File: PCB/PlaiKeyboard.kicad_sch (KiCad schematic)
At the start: 177 parts, among them SW1 SW_Push_45deg, SW10 SW_Push_45deg, SW11 SW_Push_45deg, SW12 SW_Push_45deg, SW13 SW_Push_45deg, SW14 SW_Push_45deg, SW15 RotaryEncoder_Switch, SW16 SW_Push_45deg, SW17 SW_Push_45deg, SW18 SW_Push_45deg, SW19 SW_Push_45deg, SW2 SW_Push_45deg, SW20 SW_Push_45deg, SW21 SW_Push_45deg, SW22 SW_Push_45deg, SW23 SW_Push_45deg, SW24 SW_Push_45deg, SW25 SW_Push_45deg, SW26 SW_Push_45deg, SW27 SW_Push_45deg, SW28 SW_Push_45deg, SW29 SW_Push_45deg, SW3 SW_Push_45deg, SW30 SW_Push_45deg, SW31 SW_Push_45deg, SW32 SW_Push_45deg, SW33 SW_Push_45deg, SW34 SW_Push_45deg, SW35 SW_Push_45deg, SW36 SW_Push_45deg, SW37 SW_Push_45deg, SW38 SW_Push_45deg, SW39 SW_Push_45deg, SW4 SW_Push_45deg, SW40 SW_Push_45deg, SW41 SW_Push_45deg, SW42 SW_Push_45deg, SW43 SW_Push_45deg, SW44 SW_Push_45deg, SW45 SW_Push_45deg, SW46 SW_Push_45deg, SW47 SW_Push_45deg, SW48 SW_Push_45deg, SW49 SW_Push_45deg, SW5 SW_Push_45deg, SW50 SW_Push_45deg, SW51 SW_Push_45deg, SW52 SW_Push_45deg, SW53 SW_Push_45deg, SW54 SW_Push_45deg, SW55 SW_Push_45deg, SW56 SW_Push_45deg, SW57 SW_Push_45deg, SW58 SW_Push_45deg, SW59 SW_Push_45deg, SW6 SW_Push_45deg, SW60 SW_Push_45deg, SW61 SW_Push_45deg, SW62 SW_Push_45deg, SW63 SW_Push_45deg, SW64 SW_Push_45deg, SW65 SW_Push_45deg, SW66 SW_Push_45deg, SW67 SW_Push_45deg, SW68 SW_Push_45deg, SW69 SW_Push_45deg, SW7 SW_Push_45deg, SW70 SW_Push_45deg, SW71 SW_Push_45deg, SW72 SW_Push_45deg, SW73 SW_Push_45deg, SW74 SW_Push_45deg, SW75 SW_Push_45deg, SW76 SW_Push_45deg, SW77 SW_Push_45deg, SW78 SW_Push_45deg, SW79 SW_Push_45deg, SW8 SW_Push_45deg, SW80 SW_Push_45deg, SW81 SW_Push_45deg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

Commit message: Commit
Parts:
- removed C3: 100nF, Capacitor_THT:C_Rect_L11.5mm_W5.2mm_P10.00mm_MKT, symbol Device:C
- removed D77: 1N4148, Diode_THT:D_DO-35_SOD27_P7.62mm_Horizontal, symbol Diode:1N4148
- removed SW1, SW78: SW_Push_45deg, Button_Switch_Keyboard:SW_Cherry_MX_1.00u_PCB, symbol Switch:SW_Push_45deg
- removed U2: 74HC595, Package_DIP:DIP-16_W7.62mm_LongPads, symbol 74xx:74HC595
- added D83: 1N4148, Diode_THT:D_DO-35_SOD27_P7.62mm_Horizontal, symbol Diode:1N4148
- added SW15: SW_Push_45deg, Button_Switch_Keyboard:SW_Cherry_MX_1.25u_PCB, symbol Switch:SW_Push_45deg
- added SW84: SW_Push_45deg, Button_Switch_Keyboard:SW_Cherry_MX_1.00u_PCB, symbol Switch:SW_Push_45deg
- SW22, SW8: footprint Button_Switch_Keyboard:SW_Cherry_MX_1.00u_PCB -> Button_Switch_Keyboard:SW_Cherry_MX_1.25u_PCB
- SW25: footprint Button_Switch_Keyboard:SW_Cherry_MX_1.00u_PCB -> Button_Switch_Keyboard:SW_Cherry_MX_2.00u_PCB
- SW29: footprint Button_Switch_Keyboard:SW_Cherry_MX_2.00u_PCB -> Button_Switch_Keyboard:SW_Cherry_MX_6.25u_PCB
- SW31, SW44: footprint Button_Switch_Keyboard:SW_Cherry_MX_1.50u_PCB -> Button_Switch_Keyboard:SW_Cherry_MX_1.00u_PCB
- SW39, SW47: footprint Button_Switch_Keyboard:SW_Cherry_MX_1.00u_PCB -> Button_Switch_Keyboard:SW_Cherry_MX_1.50u_PCB
- SW46, SW71: footprint Button_Switch_Keyboard:SW_Cherry_MX_1.75u_PCB -> Button_Switch_Keyboard:SW_Cherry_MX_1.00u_PCB
- SW58, SW60: footprint Button_Switch_Keyboard:SW_Cherry_MX_2.25u_PCB -> Button_Switch_Keyboard:SW_Cherry_MX_1.00u_PCB
- SW61, SW70: footprint Button_Switch_Keyboard:SW_Cherry_MX_1.00u_PCB -> Button_Switch_Keyboard:SW_Cherry_MX_1.75u_PCB
- SW62: footprint Button_Switch_Keyboard:SW_Cherry_MX_1.00u_PCB -> Button_Switch_Keyboard:SW_Cherry_MX_2.25u_PCB
- SW74, SW75: footprint Button_Switch_Keyboard:SW_Cherry_MX_1.25u_PCB -> Button_Switch_Keyboard:SW_Cherry_MX_1.00u_PCB
- SW76: footprint Button_Switch_Keyboard:SW_Cherry_MX_1.25u_PCB -> Button_Switch_Keyboard:SW_Cherry_MX_2.25u_PCB
- SW77: footprint Button_Switch_Keyboard:SW_Cherry_MX_6.25u_PCB -> Button_Switch_Keyboard:SW_Cherry_MX_1.00u_PCB
- renumbered C2 to C1, C1 to C2, D83 to D77, SW84 to SW1, SW15 to SW78
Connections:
- net SR_CLOCK is gone; now on net ROW0: U1.5 (P0.17)
- net SR_DATA is gone; now on net ROW1: U1.6 (P0.20)
- net SR_LATCH is gone; now on net ROW2: U1.7 (P0.22)
- net COL0: now also SW2.1, SW3.1, SW4.1, SW5.1, SW6.1, SW7.1, SW8.1, U1.12 (P1.06-LF); no longer SW16.1, SW31.1, SW46.1, SW60.1, SW74.1, U1.26 (P1.02-LF)
- net COL1: now also SW10.1, SW11.1, SW12.1, SW13.1, SW14.1, SW9.1, U1.25 (P1.01-LF), SW15.1; no longer SW17.1, SW2.1, SW32.1, SW47.1, SW61.1, SW75.1, U1.27 (P1.07-LF)
- net COL10: now also SW72.1, SW73.1, SW74.1, SW75.1, SW76.1, SW77.1, SW78.S2, U1.23 (P0.10-LF); no longer SW11.1, SW26.1, SW41.1, SW56.1, SW70.1
- net COL11: now also SW79.1, SW80.1, SW81.1, SW82.1, SW83.1, U1.24 (P0.09-LF), SW84.1; no longer SW12.1, SW27.1, SW42.1, SW57.1, SW71.1
- net COL2: now also SW16.1, SW17.1, SW19.1, SW20.1, SW21.1, SW22.1, U1.26 (P1.02-LF); no longer SW3.1, SW33.1, SW48.1, SW62.1, SW76.1, U1.17 (P0.31-LF)
- net COL3: now also SW23.1, SW24.1, SW25.1, SW26.1, SW27.1, SW28.1, SW29.1, U1.27 (P1.07-LF); no longer SW19.1, SW34.1, SW4.1, SW49.1, SW63.1, SW77.1, U1.18 (P0.29-LF)
- net COL4: now also SW30.1, SW31.1, SW32.1, SW33.1, SW34.1, SW36.1, U1.17 (P0.31-LF); no longer SW20.1, SW5.1, SW50.1, SW64.1, U1.19 (P0.02-LF)
- net COL5: now also SW37.1, SW38.1, SW39.1, SW40.1, SW41.1, SW42.1, SW43.1, U1.18 (P0.29-LF); no longer SW21.1, SW36.1, SW51.1, SW6.1, SW65.1, SW79.1, U1.20 (P1.15-LF)
- net COL6: now also SW44.1, SW45.1, SW46.1, SW47.1, SW48.1, SW49.1, SW50.1, U1.19 (P0.02-LF); no longer SW22.1, SW37.1, SW52.1, SW66.1, SW7.1, SW80.1, U1.21 (P1.13-LF)
- net COL7: now also SW51.1, SW52.1, SW54.1, SW55.1, SW56.1, SW57.1, U1.20 (P1.15-LF); no longer SW23.1, SW38.1, SW67.1, SW8.1, SW81.1, U1.22 (P1.11-LF)
- net COL8: now also SW58.1, SW59.1, SW60.1, SW61.1, SW62.1, SW63.1, SW64.1, U1.21 (P1.13-LF); no longer SW24.1, SW39.1, SW54.1, SW68.1, SW82.1, SW9.1, U1.23 (P0.10-LF)
- net COL9: now also SW65.1, SW66.1, SW67.1, SW68.1, SW70.1, SW71.1, U1.22 (P1.11-LF); no longer SW10.1, SW25.1, SW40.1, SW55.1, SW83.1, U1.24 (P0.09-LF)
- net ROW0: now also D15.1 (K), D22.1 (K), D29.1 (K), D36.1 (K), D43.1 (K), D50.1 (K), D57.1 (K), D64.1 (K), D71.1 (K), D78.1 (K); no longer D10.1 (K), D11.1 (K), D12.1 (K), D13.1 (K), D14.1 (K), D2.1 (K), D3.1 (K), D4.1 (K), D5.1 (K), D6.1 (K), D7.1 (K), D77.1 (K), D9.1 (K), U1.8 (P0.24)
- net ROW1: now also D2.1 (K), D30.1 (K), D37.1 (K), D44.1 (K), D51.1 (K), D58.1 (K), D65.1 (K), D72.1 (K), D79.1 (K), D9.1 (K); no longer D15.1 (K), D17.1 (K), D18.1 (K), D19.1 (K), D20.1 (K), D21.1 (K), D22.1 (K), D24.1 (K), D25.1 (K), D26.1 (K), D27.1 (K), D28.1 (K), D29.1 (K), U1.9 (P1.00)
- net ROW2: now also D10.1 (K), D17.1 (K), D24.1 (K), D3.1 (K), D45.1 (K), D52.1 (K), D59.1 (K), D66.1 (K), D73.1 (K), D80.1 (K); no longer D30.1 (K), D32.1 (K), D33.1 (K), D34.1 (K), D35.1 (K), D36.1 (K), D37.1 (K), D39.1 (K), D40.1 (K), D41.1 (K), D42.1 (K), D43.1 (K), D44.1 (K), U1.10 (P0.11)
- net ROW3: now also D11.1 (K), D18.1 (K), D25.1 (K), D32.1 (K), D39.1 (K), D4.1 (K), D60.1 (K), D67.1 (K), D74.1 (K), D81.1 (K), U1.8 (P0.24); no longer D45.1 (K), D47.1 (K), D48.1 (K), D49.1 (K), D50.1 (K), D51.1 (K), D52.1 (K), D54.1 (K), D55.1 (K), D56.1 (K), D57.1 (K), D58.1 (K), U1.11 (P1.04-LF)
- net ROW4: now also D12.1 (K), D19.1 (K), D26.1 (K), D33.1 (K), D40.1 (K), D47.1 (K), D5.1 (K), D54.1 (K), D75.1 (K), D82.1 (K), U1.9 (P1.00); no longer D59.1 (K), D60.1 (K), D62.1 (K), D63.1 (K), D64.1 (K), D65.1 (K), D66.1 (K), D67.1 (K), D69.1 (K), D70.1 (K), D71.1 (K), D72.1 (K), U1.12 (P1.06-LF)
- net ROW5: now also D13.1 (K), D20.1 (K), D27.1 (K), D34.1 (K), D41.1 (K), D48.1 (K), D55.1 (K), D6.1 (K), D62.1 (K), D69.1 (K), U1.10 (P0.11), D83.1 (K); no longer D73.1 (K), D74.1 (K), D75.1 (K), D78.1 (K), D79.1 (K), D80.1 (K), D81.1 (K), D82.1 (K), U1.25 (P1.01-LF)
- net at SW11.2: now also D10.2 (A); no longer D11.2 (A)
- net at SW5.2: now also D4.2 (A); no longer D5.2 (A)
- net at D6.2 (A): now also SW7.2; no longer SW6.2
- net at D9.2 (A): now also SW10.2; no longer SW9.2
- net at D14.2 (A): now also SW15.2; no longer SW14.2
- net at SW12.2: now also D11.2 (A); no longer D12.2 (A)
- net at D1.2 (A): now also SW2.2
- net at D8.2 (A): now also SW9.2; no longer SW8.2
- net at D7.2 (A): now also SW8.2; no longer SW7.2
- net at SW4.2: now also D3.2 (A); no longer D4.2 (A)
- net at D2.2 (A): now also SW3.2; no longer SW2.2
- net at SW13.2: now also D12.2 (A); no longer D13.2 (A)
- removed net COL12: SW13.1, SW28.1, SW43.1, SW58.1, SW72.1
- removed net COL13: SW14.1, SW29.1, SW44.1, SW59.1, SW73.1
- removed net COL14: SW30.1, SW45.1, SW78.S2
- new net: D83.2 (A), SW84.2
- new net: D5.2 (A), SW6.2
- new net: D13.2 (A), SW14.2
- new net ROW6: D14.1 (K), D21.1 (K), D28.1 (K), D35.1 (K), D42.1 (K), D49.1 (K), D56.1 (K), D63.1 (K), D7.1 (K), D70.1 (K), D77.1 (K), U1.11 (P1.04-LF)
- no-connect marks 5 -> 1
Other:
- moved on the sheet: C1, C2, D77, J_BAT1, S1, S2, S3, S4, SW1, SW78, U1

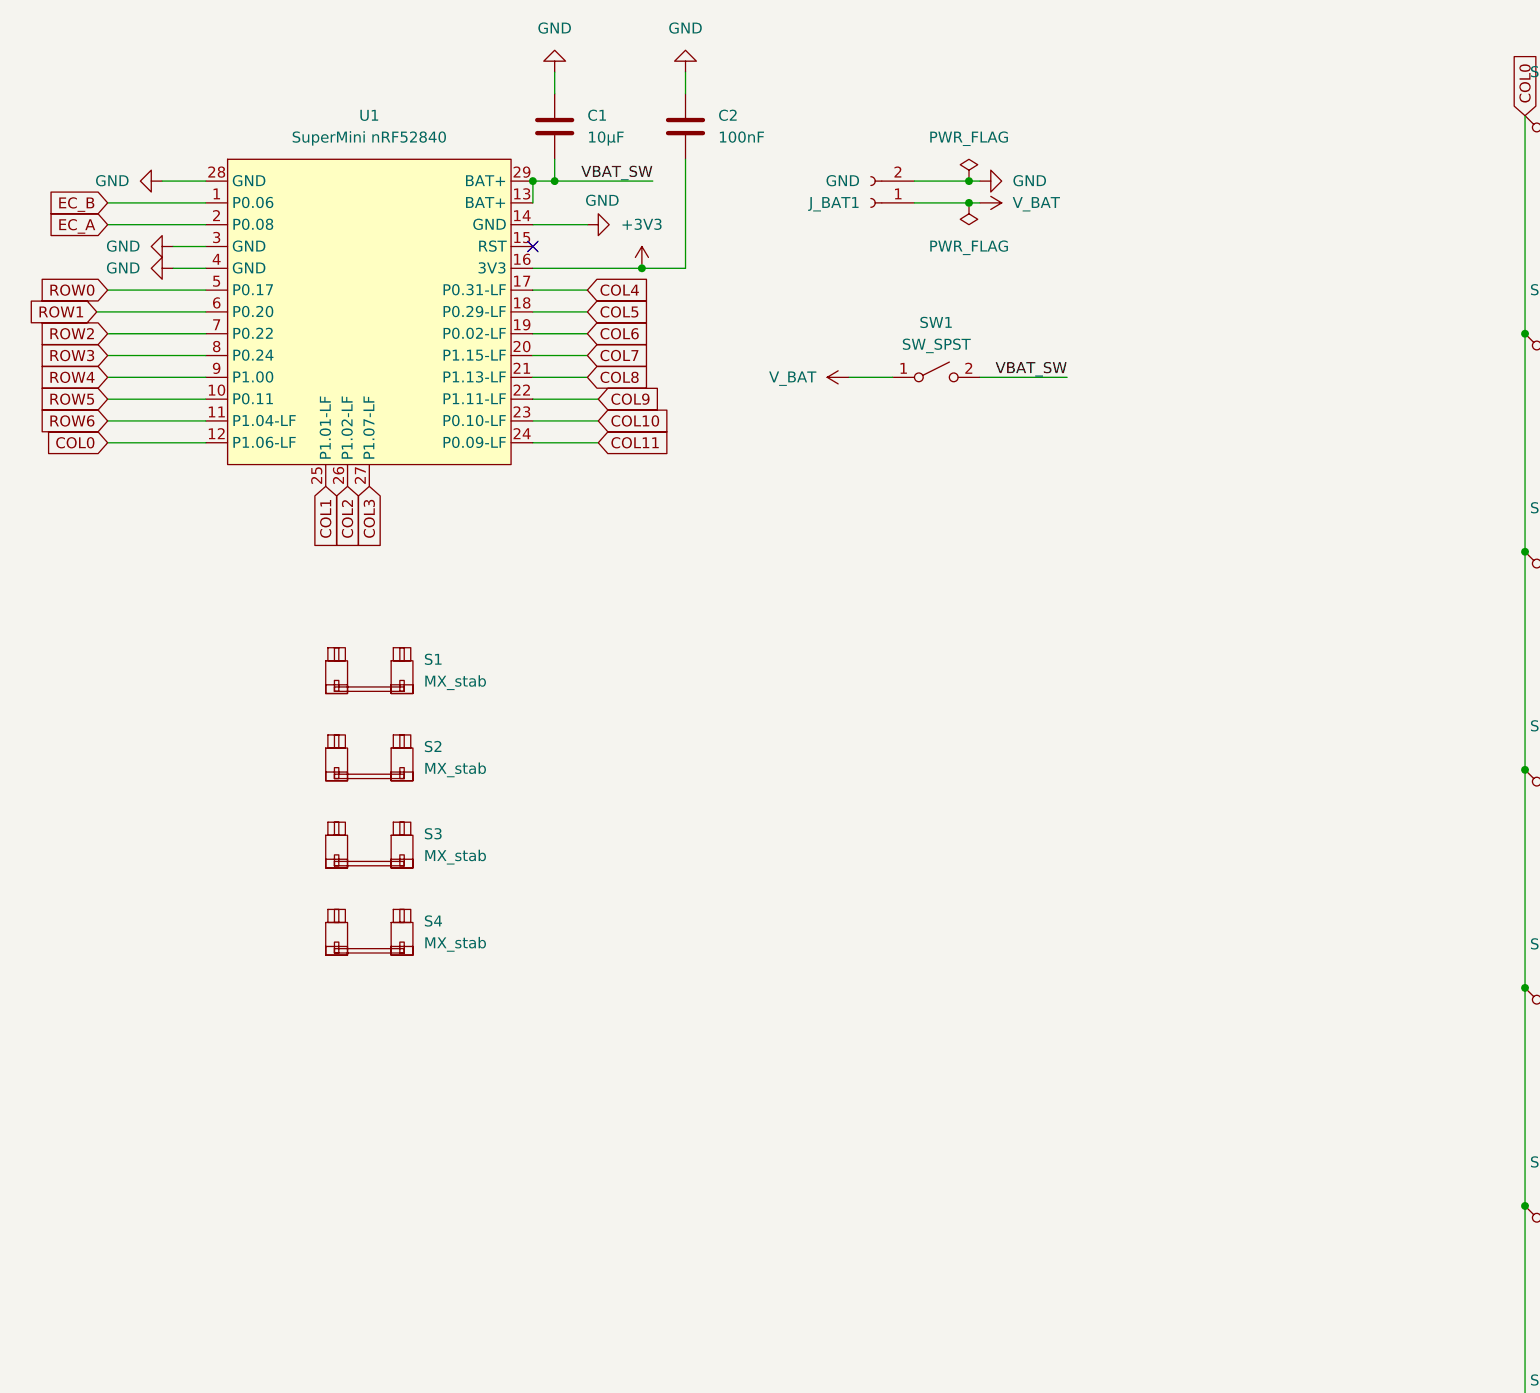
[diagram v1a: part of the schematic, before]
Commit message: New Changes
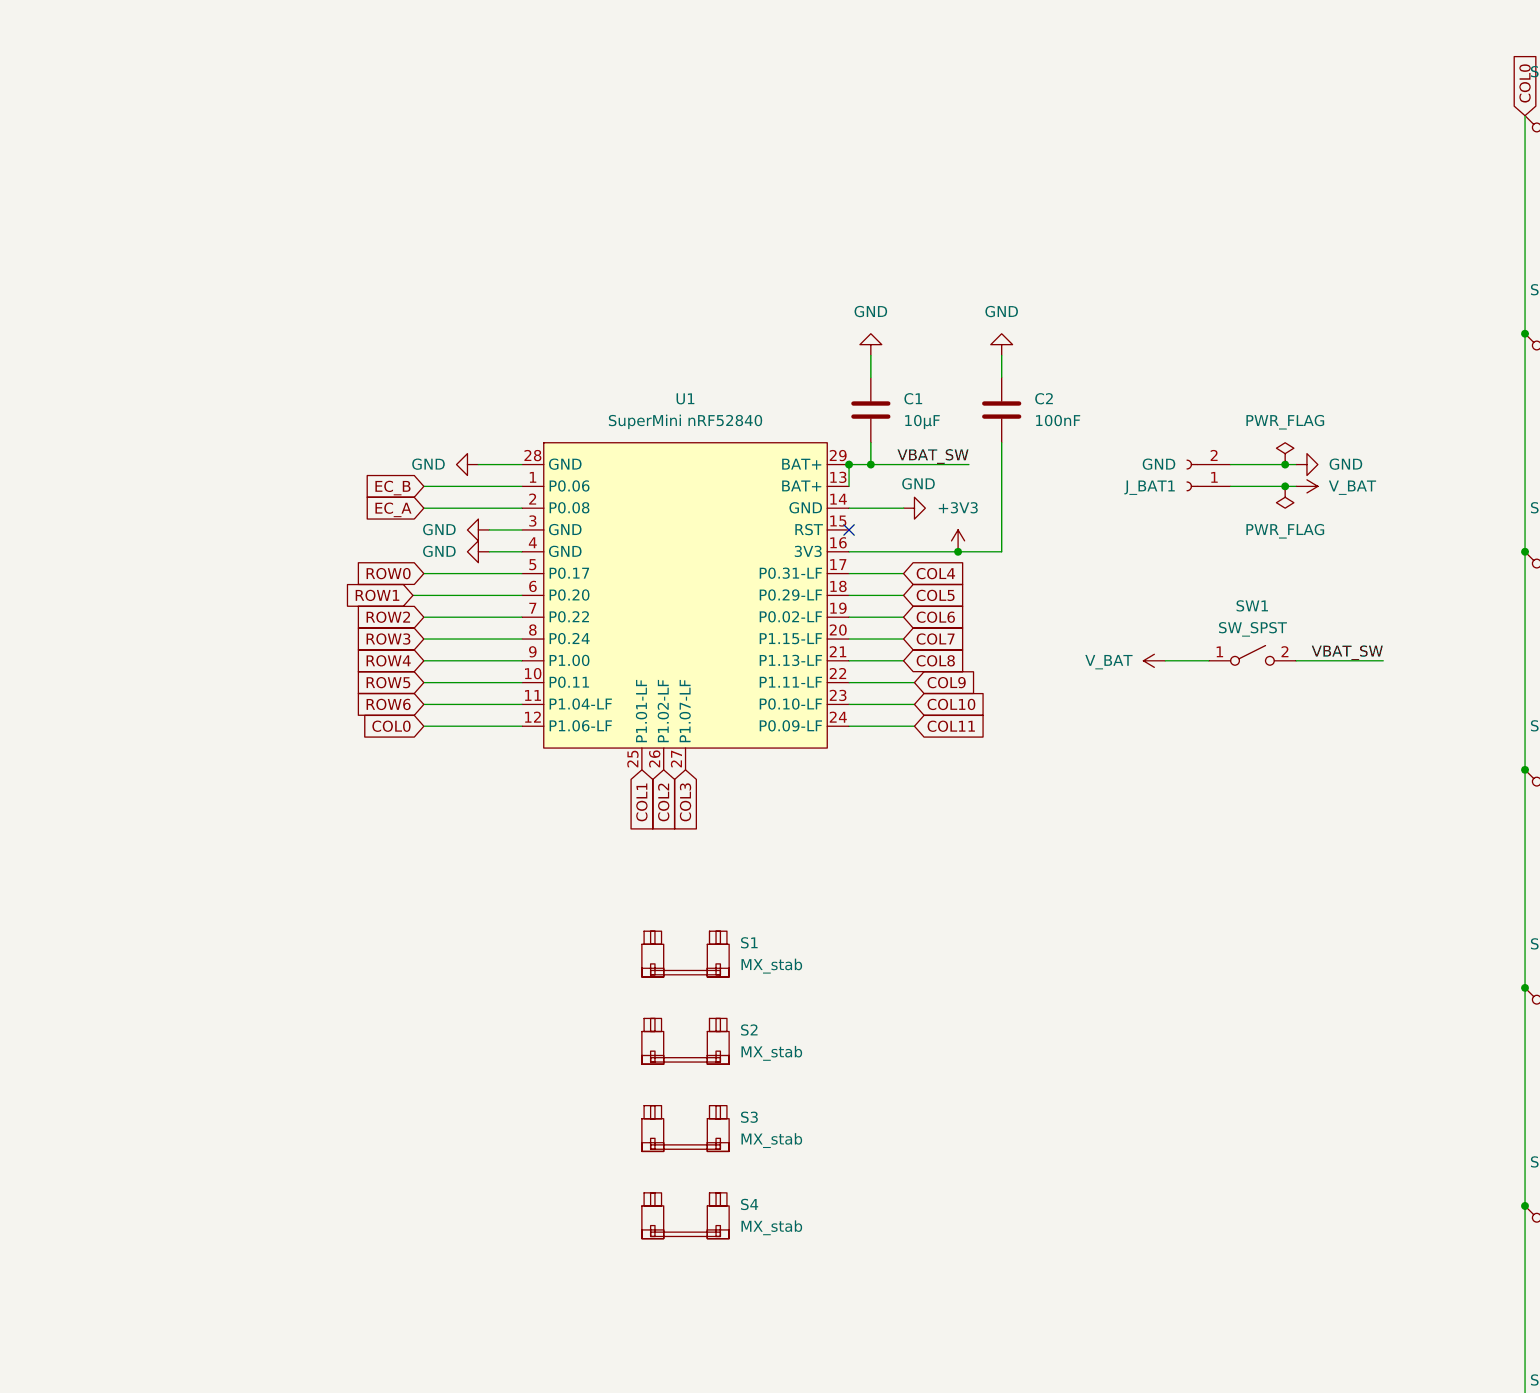
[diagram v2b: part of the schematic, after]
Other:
- moved on the sheet: C1, C2, J_BAT1, S1, S2, S3, S4, SW1, U1
